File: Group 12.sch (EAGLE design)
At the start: 30 parts, among them U1 328P, Y1 16MHz

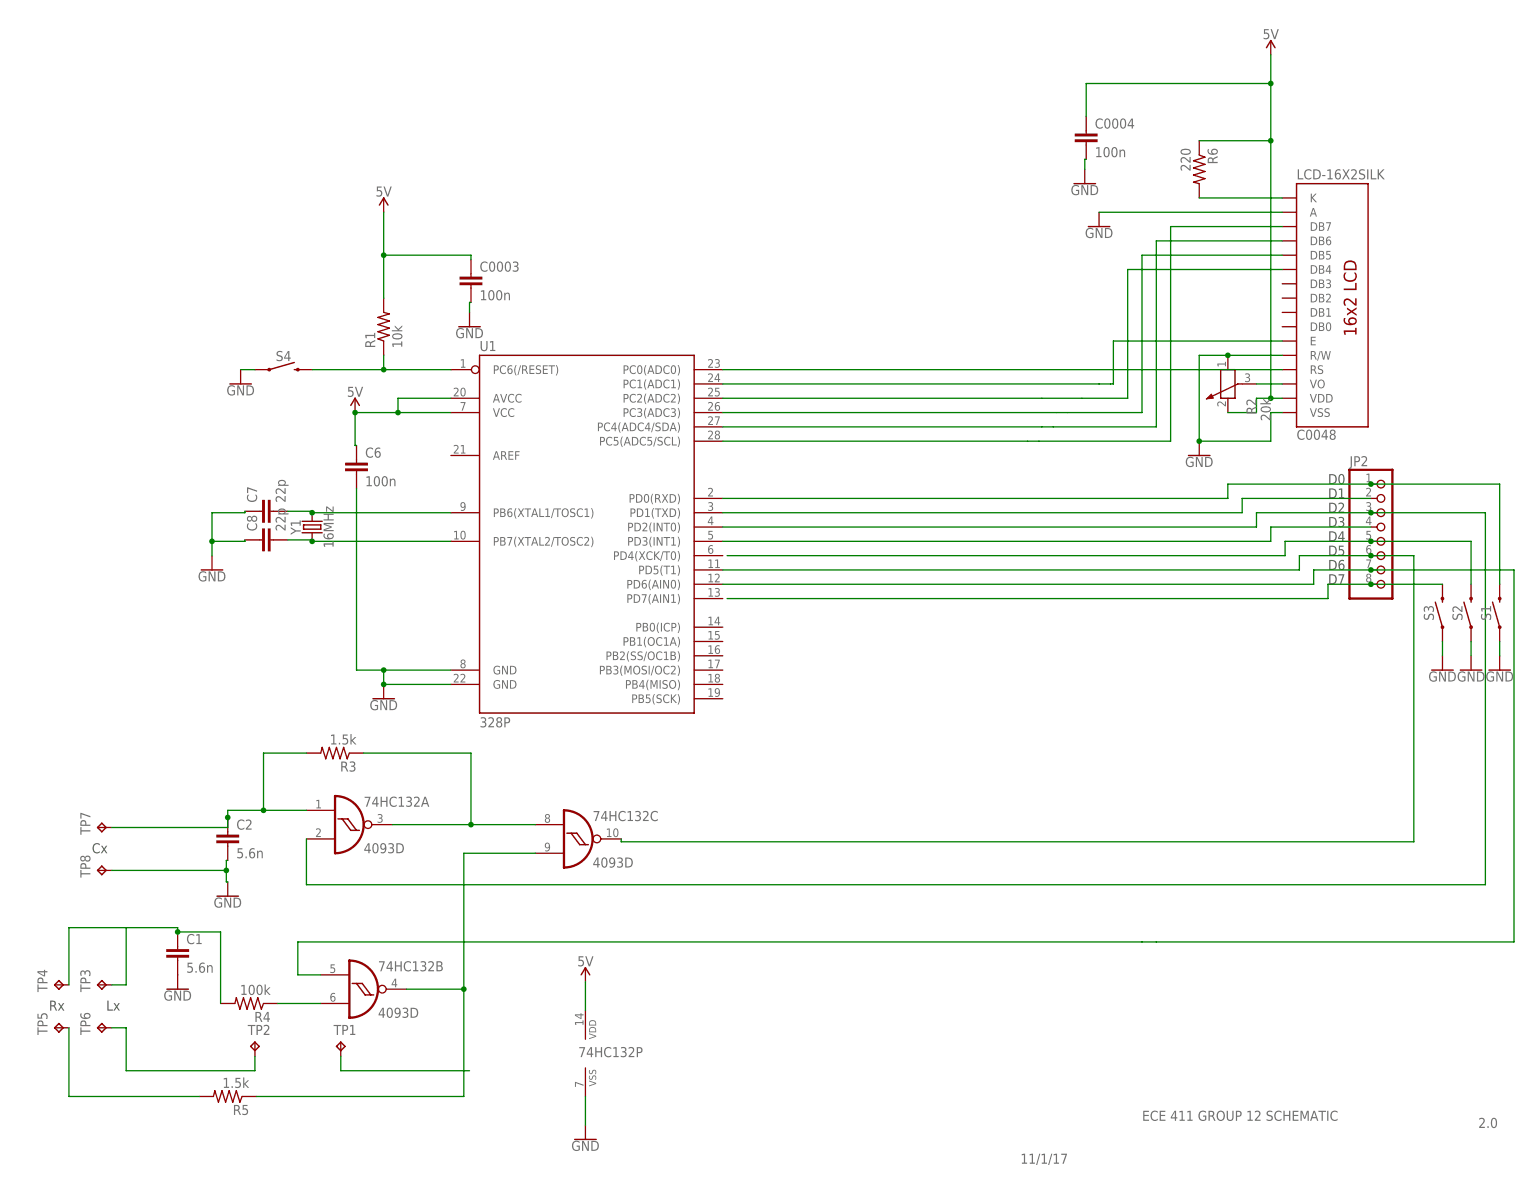
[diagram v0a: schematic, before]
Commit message: board and sch
board and sch
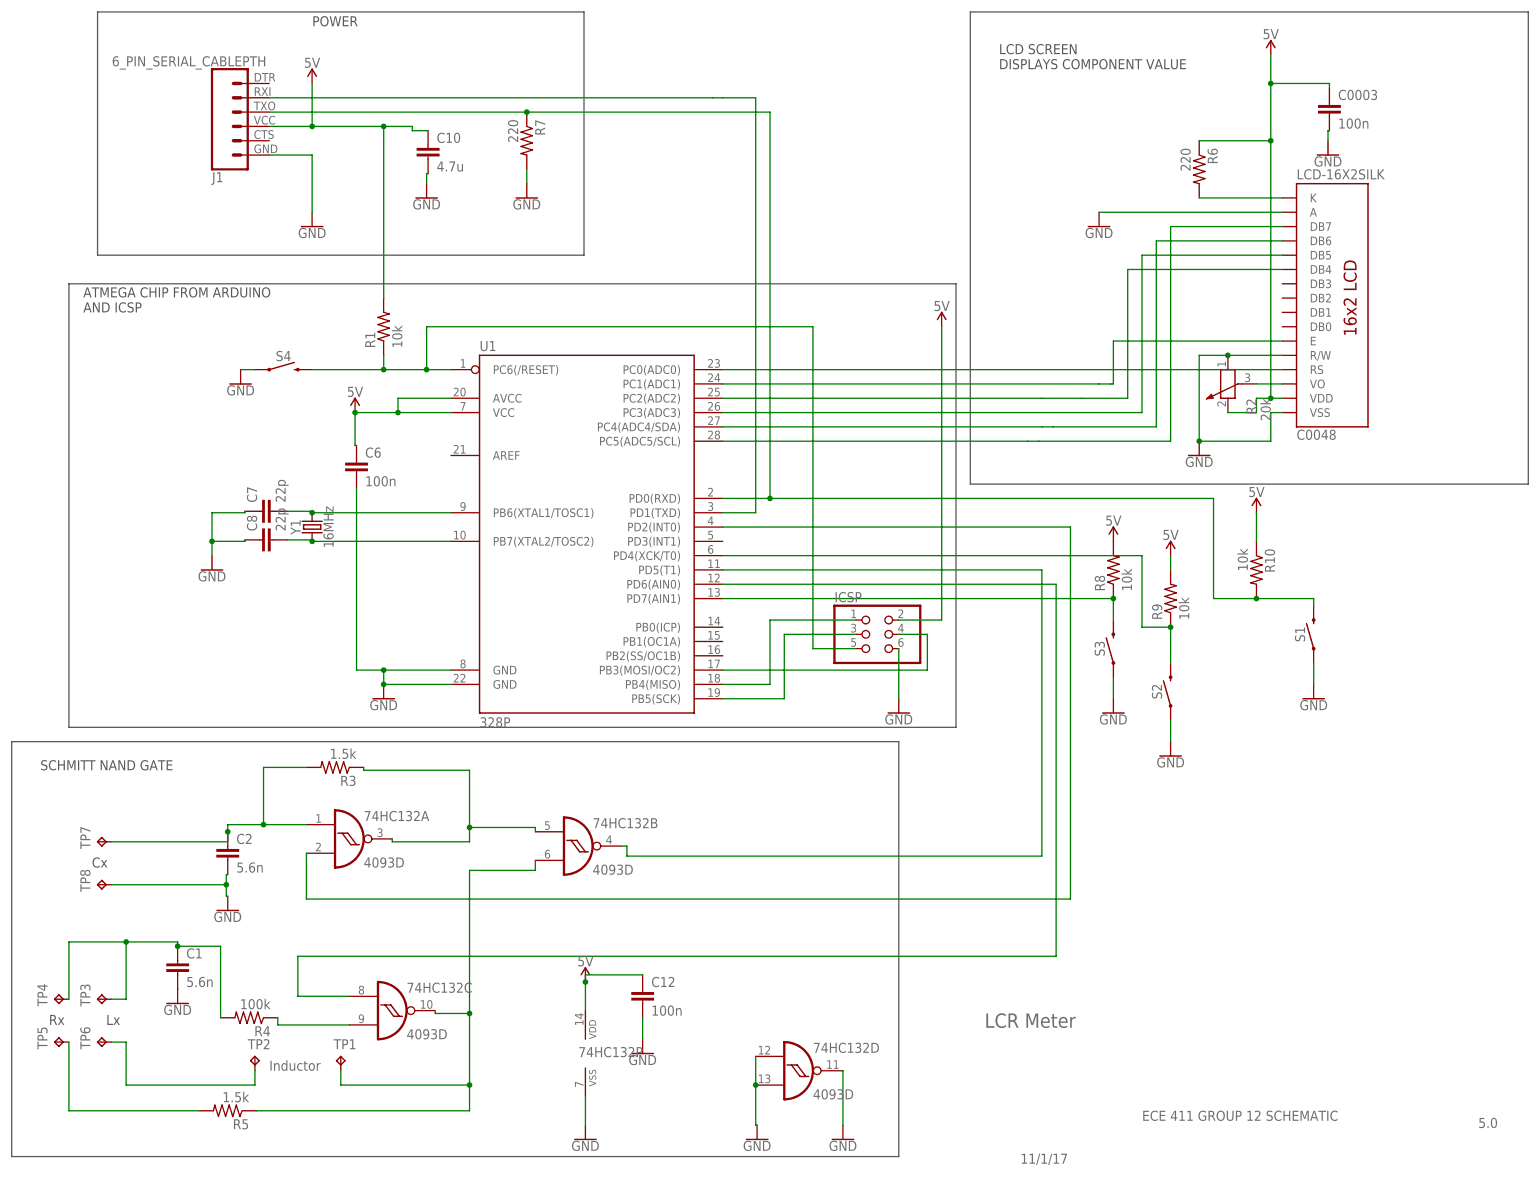
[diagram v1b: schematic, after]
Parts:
- removed C0004: 100n, rcl:C-EUC0805K
- removed JP2: (no value), pinhead:PINHD-1X8
- added C10: 4.7u, rcl:C-EUC0805K
- added C12: 100n, rcl:C-EUC0805K
- added ICSP: (no value), pinhead:PINHD-2X3
- added J1: 6_PIN_SERIAL_CABLEPTH, SparkFun-Connectors:6_PIN_SERIAL_CABLEPTH
- added R10, R8, R9: 10k, rcl:R-US_R0805
- added R7: 220, rcl:R-US_R0805
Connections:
- net N$21 renamed PC0
- net N$24 renamed PB6
- net N$25 renamed PB7
- net N$4 renamed PC1
- net N$5 renamed PC2
- net N$6 renamed PC3
- net N$7 renamed PC4
- net N$8 renamed PC5
- removed net N$11: 74HC132B.I1, R4.1
- removed net N$12: C1.1, R4.2, TP4.TP
- removed net N$13: TP1.TP
- removed net N$15: R1.1, S4.2, U1.PC6(/RESET)
- removed net N$18: 74HC132B.I0, JP2.7, U1.PD6(AIN0)
- removed net N$35: 74HC132C.O, JP2.6, U1.PD5(T1)
- removed net N$36: JP2.4, U1.PD3(INT1)
- removed net N$37: JP2.5, S2.2
- removed net N$39: JP2.2, U1.PD1(TXD)
- removed net N$40: JP2.1, S1.2, U1.PD0(RXD)
- removed net N$9: 74HC132A.O, 74HC132C.I0, R3.1
- new net CAL: R9.1, S2.2, U1.PD4(XCK/T0)
- new net MISO: ICSP.1, U1.PB4(MISO)
- new net N$4: ICSP.4, U1.PB3(MOSI/OC2)
- new net N$5: 74HC132A.O, 74HC132B.I0, R3.1
- new net PD0: J1.3, R10.2, R7.1, S1.2, U1.PD0(RXD)
- new net PD2: 74HC132A.I1, U1.PD2(INT0)
- new net PD5: 74HC132B.O, U1.PD5(T1)
- new net PD6: 74HC132C.I0, U1.PD6(AIN0)
- new net RESET: ICSP.5, R1.1, S4.2, U1.PC6(/RESET)
- new net SCK: ICSP.3, U1.PB5(SCK)
- new net SET: R8.1, S3.2, U1.PD7(AIN1)
- net 5V: now also C10.1, C12.1, ICSP.2, J1.4, R10.1, R8.2, R9.2; no longer C0004.1
- net GND: now also 74HC132D.I0, 74HC132D.I1, 74HC132D.O, C10.2, C12.2, ICSP.6, J1.6, R7.2; no longer C0004.2
- net N$1: now also 74HC132C.I1, R4.1; no longer JP2.8, S3.2
- net N$10: now also 74HC132B.I1, 74HC132C.O, TP1.TP; no longer 74HC132B.O, 74HC132C.I1
- net N$16: now also C1.1, R4.2, TP4.TP
- net N$3: now also J1.2, U1.PD1(TXD); no longer 74HC132A.I1, JP2.3, U1.PD2(INT0)
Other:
- note added: "5.0"
- note added: "ATMEGA CHIP FROM ARDUINO AND ICSP"
- note added: "Inductor"
- note added: "LCD SCREEN DISPLAYS COMPONENT VALUE"
- note added: "LCR Meter"
- note added: "POWER"
- note added: "SCHMITT NAND GATE"
- note removed: "2.0"
- note removed: "D0"
- note removed: "D1"
- note removed: "D2"
- note removed: "D3"
- note removed: "D4"
- note removed: "D5"
- note removed: "D6"
- note removed: "D7"
- moved on the sheet: 74HC132A, 74HC132B, 74HC132C, C0003, C1, C2, R3, R4, R5, S1, S2, S3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
